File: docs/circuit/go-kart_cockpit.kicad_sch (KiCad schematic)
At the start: 40 parts, among them P1 LED, Q1 IRLIZ44N, X1 Taster rechts (male), X10 Display (male), X11 PD7, X12 SDA PG4, X13 AVR-ISP-10, X14 Taster links (male), X15 Start/Stop/Rückwärts, X2 5V GND, X3 24V Hupe, X4 SCL, X5 CS, X6 PB6, X7 J5, X8 J3, X9 Bluetooth-Modul

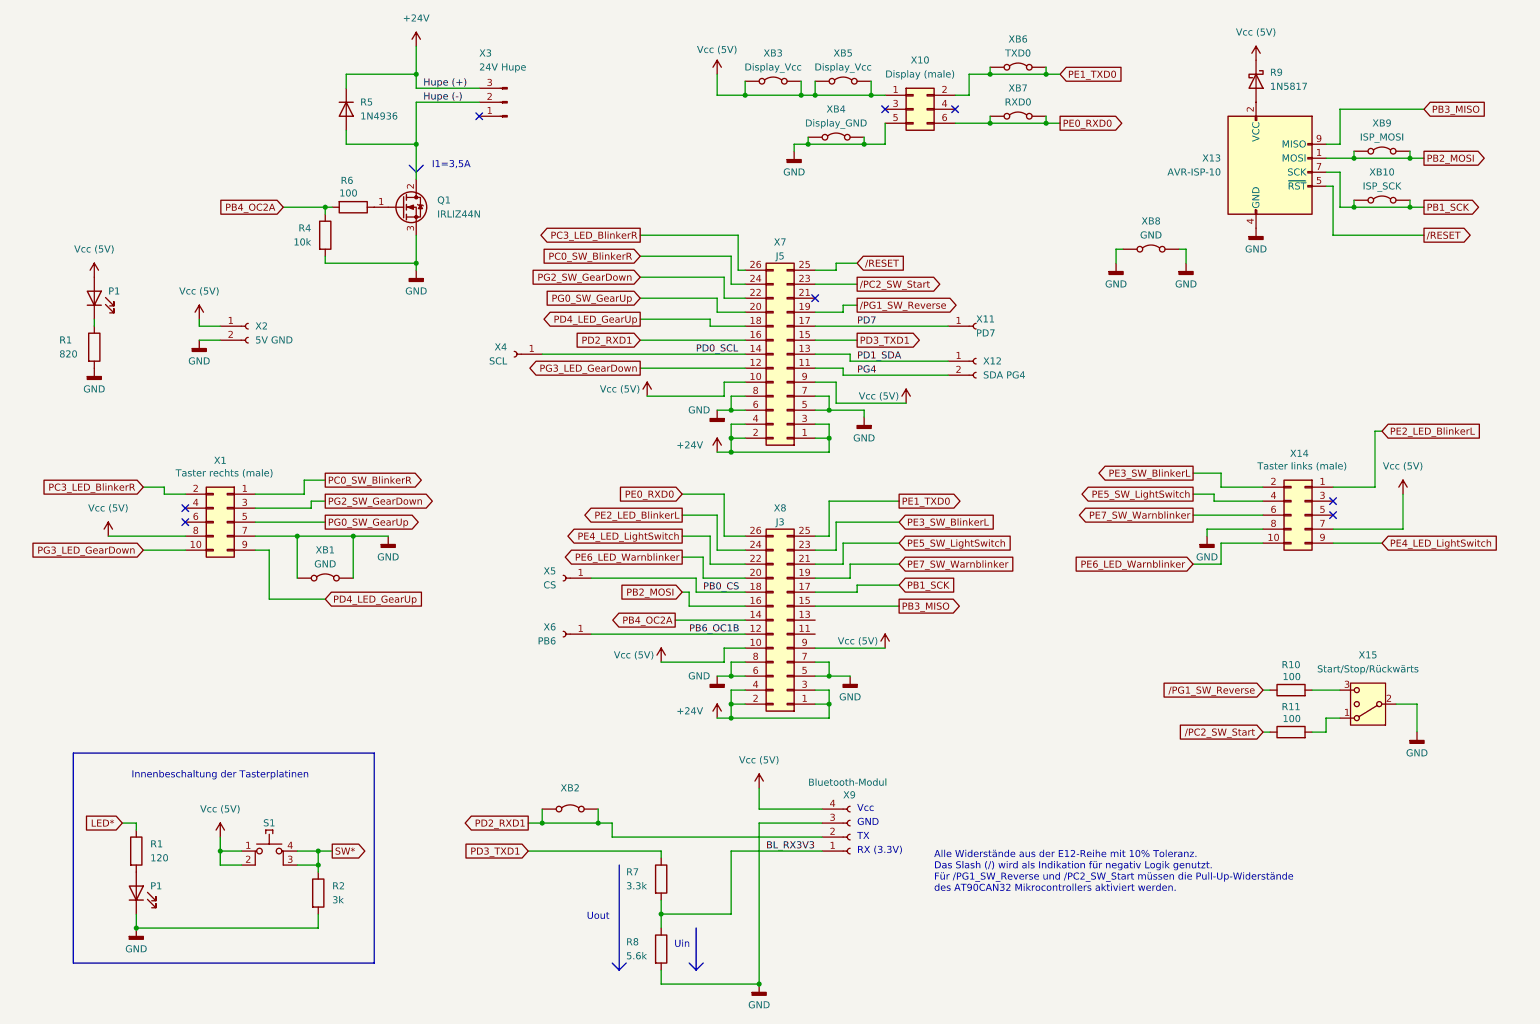
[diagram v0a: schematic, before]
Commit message: feat: rework of PCB, fix wrong connection
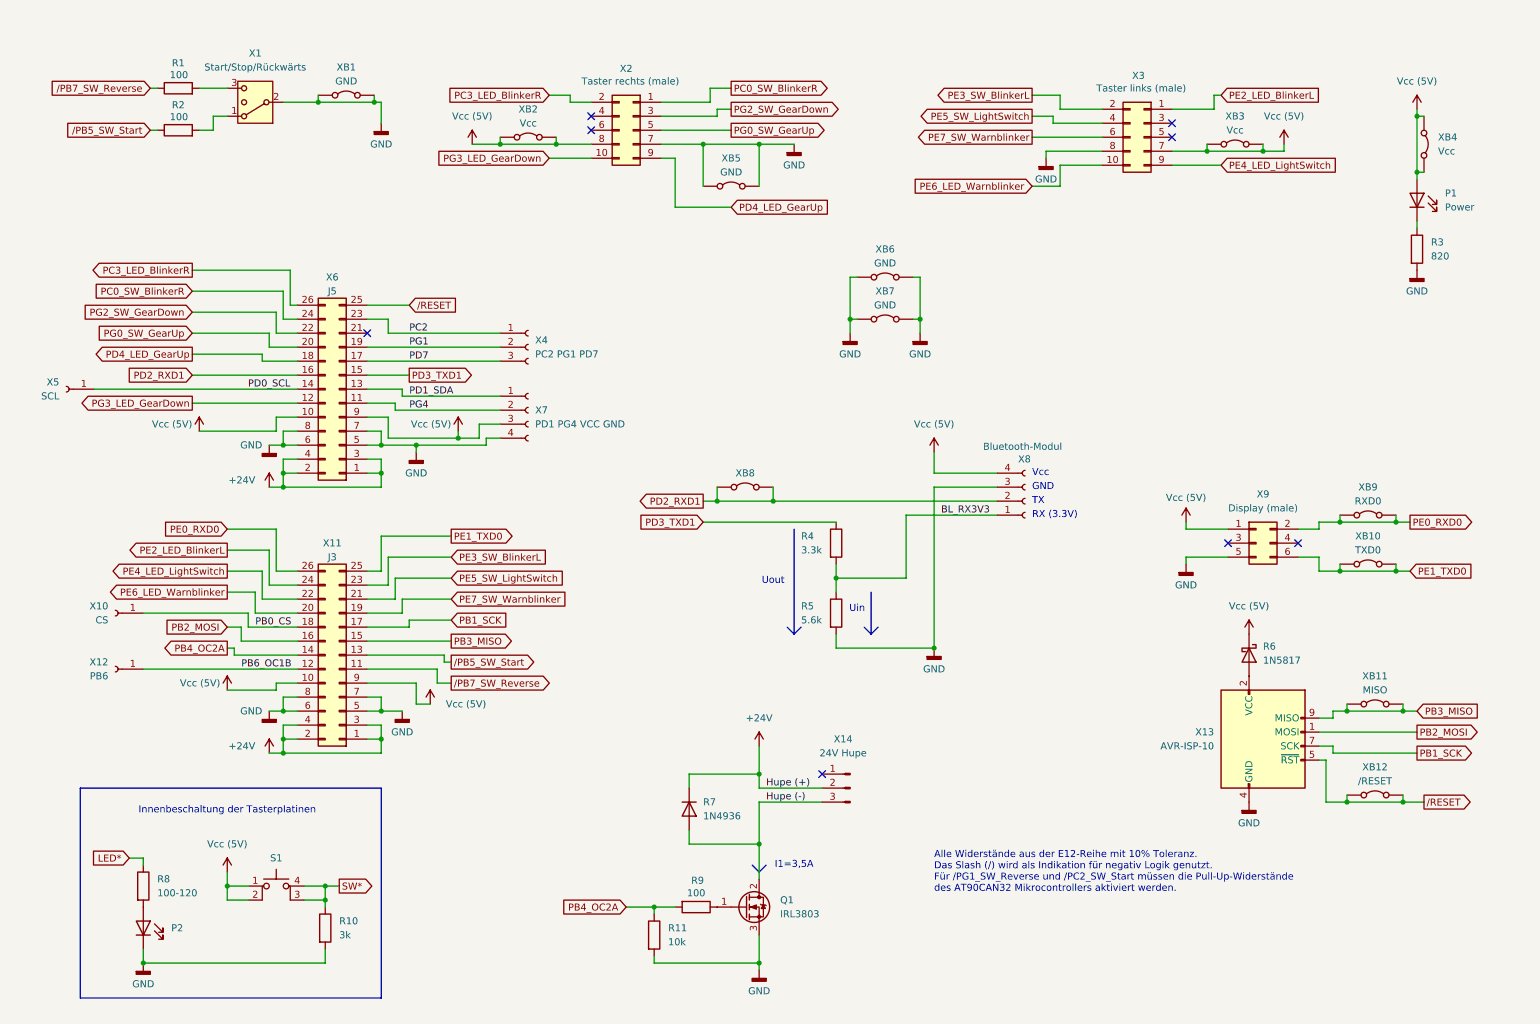
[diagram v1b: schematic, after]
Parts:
- removed P1: LED, symbol Device:LED
- removed X11: PD7, Connector_PinSocket_2.54mm:PinSocket_1x01_P2.54mm_Vertical, symbol Connector:Conn_01x01_Socket
- removed X12: SDA PG4, Connector_PinSocket_2.54mm:PinSocket_1x02_P2.54mm_Vertical, symbol Connector:Conn_01x02_Socket
- removed X2: 5V GND, Connector_PinSocket_2.54mm:PinSocket_1x02_P2.54mm_Vertical, symbol Connector:Conn_01x02_Socket
- removed XB10: ISP_SCK, Resistor_THT:R_Axial_DIN0207_L6.3mm_D2.5mm_P10.16mm_Horizontal, symbol Jumper:Jumper_2_Bridged
- removed XB4: Display_GND, Resistor_THT:R_Axial_DIN0207_L6.3mm_D2.5mm_P10.16mm_Horizontal, symbol Jumper:Jumper_2_Bridged
- removed XB5: Display_Vcc, Resistor_THT:R_Axial_DIN0207_L6.3mm_D2.5mm_P15.24mm_Horizontal, symbol Jumper:Jumper_2_Bridged
- removed XB9: ISP_MOSI, Resistor_THT:R_Axial_DIN0207_L6.3mm_D2.5mm_P15.24mm_Horizontal, symbol Jumper:Jumper_2_Bridged
- added P2: Power, LED_THT:LED_D3.0mm_Horizontal_O1.27mm_Z6.0mm, symbol Device:LED
- added X4: PC2 PG1 PD7, Connector_PinSocket_2.54mm:PinSocket_1x03_P2.54mm_Vertical, symbol Connector:Conn_01x03_Socket
- added X7: PD1 PG4 VCC GND, Connector_PinSocket_2.54mm:PinSocket_1x04_P2.54mm_Vertical, symbol Connector:Conn_01x04_Socket
- added XB1, XB6: GND, Resistor_THT:R_Axial_DIN0207_L6.3mm_D2.5mm_P10.16mm_Horizontal, symbol Jumper:Jumper_2_Bridged
- added XB11: MISO, TestPoint:TestPoint_2Pads_Pitch5.08mm_Drill1.3mm, symbol Jumper:Jumper_2_Bridged
- added XB12: /RESET, Resistor_THT:R_Axial_DIN0207_L6.3mm_D2.5mm_P15.24mm_Horizontal, symbol Jumper:Jumper_2_Bridged
- added XB2, XB3: Vcc, Resistor_THT:R_Axial_DIN0207_L6.3mm_D2.5mm_P10.16mm_Horizontal, symbol Jumper:Jumper_2_Bridged
- P1: value LED -> Power; footprint (none) -> LED_THT:LED_D3.0mm_Horizontal_O1.27mm_Z6.0mm
- Q1: value IRLIZ44N -> IRL3803; footprint Library:TO-220-3_Horizontal_TabDown_no_hole -> Package_TO_SOT_THT:TO-220F-3_Horizontal_TabDown
- R3: renamed from R1; footprint Resistor_THT:R_Axial_DIN0207_L6.3mm_D2.5mm_P10.16mm_Horizontal -> Resistor_THT:R_Axial_DIN0309_L9.0mm_D3.2mm_P12.70mm_Horizontal
- R4: renamed from R7; footprint Resistor_THT:R_Axial_DIN0207_L6.3mm_D2.5mm_P15.24mm_Horizontal -> Resistor_THT:R_Axial_DIN0207_L6.3mm_D2.5mm_P10.16mm_Horizontal
- R8: renamed from R1; value 120 -> 100-120; now in the parts list
- R9: renamed from R6; footprint Resistor_THT:R_Axial_DIN0309_L9.0mm_D3.2mm_P25.40mm_Horizontal -> Resistor_THT:R_Axial_DIN0207_L6.3mm_D2.5mm_P7.62mm_Horizontal
- XB4: renamed from XB3; value Display_Vcc -> Vcc
- renumbered R10 to R1, R2 to R10, R4 to R11, R11 to R2, R8 to R5, R9 to R6, R5 to R7, X15 to X1, X5 to X10, X8 to X11, X6 to X12, X3 to X14, X1 to X2, X14 to X3, X4 to X5, X7 to X6, X9 to X8, X10 to X9, XB6 to XB10, XB8 to XB5, XB1 to XB7, XB2 to XB8, XB7 to XB9
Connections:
- net +24V: now also X14.2 (Pin_2); no longer X14.3 (Pin_3)
- net GND: now also P2.1 (K), X7.4 (Pin_4), XB1.1 (A), XB1.2 (B), XB6.1 (A), XB6.2 (B)
- net Hupe (-): now also X14.3 (Pin_3); no longer X14.2 (Pin_2)
- net PB3_MISO: now also XB11.1 (A), XB11.2 (B)
- net PD1_SDA: now also X7.1 (Pin_1)
- net PD7: now also X4.3 (Pin_3)
- net PE0_RXD0: now also X9.2 (Pin_2); no longer X9.6 (Pin_6)
- net PE1_TXD0: now also X9.6 (Pin_6); no longer X9.2 (Pin_2)
- net PG4: now also X7.2 (Pin_2)
- net Vcc (5V): now also X7.3 (Pin_3), XB2.1 (A), XB2.2 (B), XB3.1 (A), XB3.2 (B)
- net /RESET: now also XB12.1 (A), XB12.2 (B)
- net at R8.2: now also P2.2 (A)
- net /PB7_SW_Reverse: now reaches X11.11 (Pin_11)
- net /PB7_SW_Reverse: now also R1.1
- net /PB5_SW_Start: now reaches X11.13 (Pin_13)
- net /PB5_SW_Start: now also R2.1
- net /PC2_SW_Start renamed PC2
- net PC2: now also X4.1 (Pin_1); no longer R2.1
- net /PG1_SW_Reverse renamed PG1
- net PG1: now also X4.2 (Pin_2); no longer R1.1
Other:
- moved on the sheet: P1, Q1, R1, R10, R11, R2, R3, R4, R5, R6, R7, R8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
